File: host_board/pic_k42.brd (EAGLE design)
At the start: 55.6 x 67.3 mm, 40 parts, among them IC1 PIC18F57K42-E_PT, IC2 REF3440IDBVR, IC3 MAX232, K1 G6K-2P, Q1 ASF1, X1 332-02, X2 332-02, X3 332-02, X4 22-23-2101, X5 22-23-2101, X6 22-23-2101, X7 22-23-2101

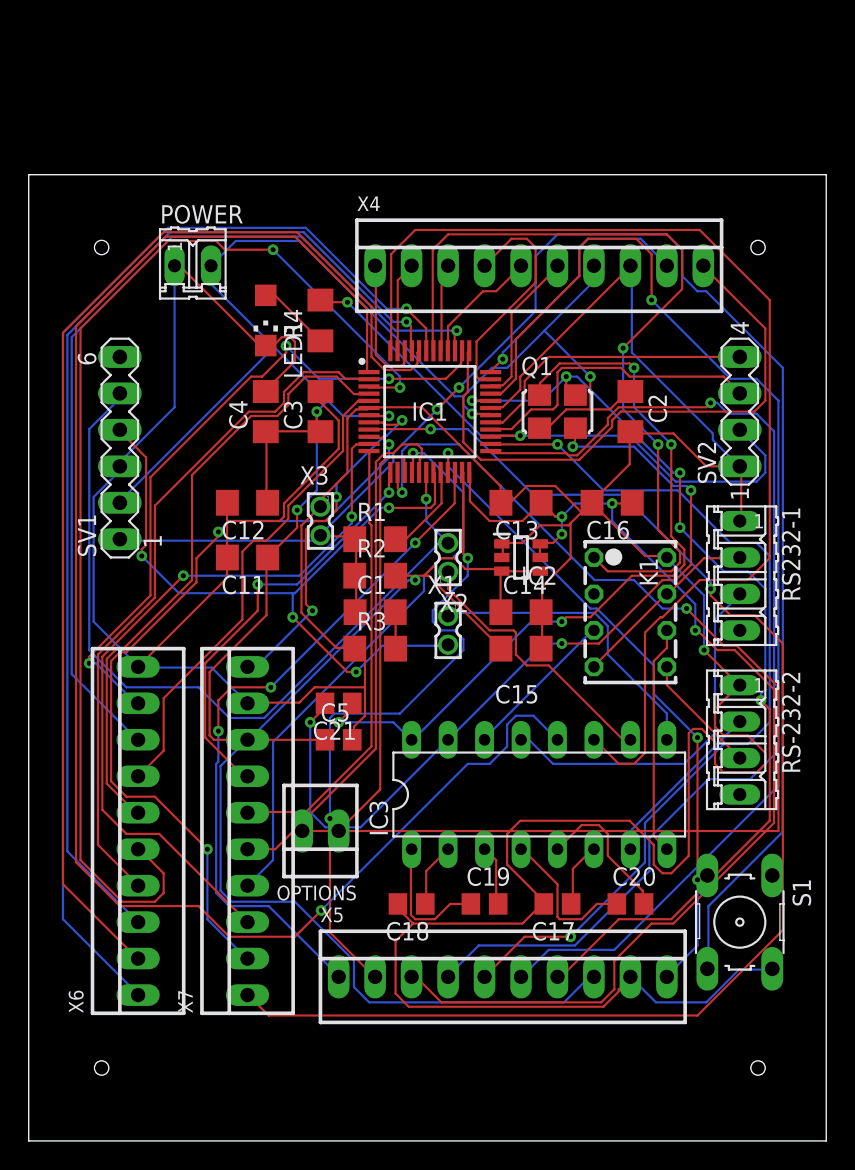
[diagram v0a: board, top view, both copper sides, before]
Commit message: update
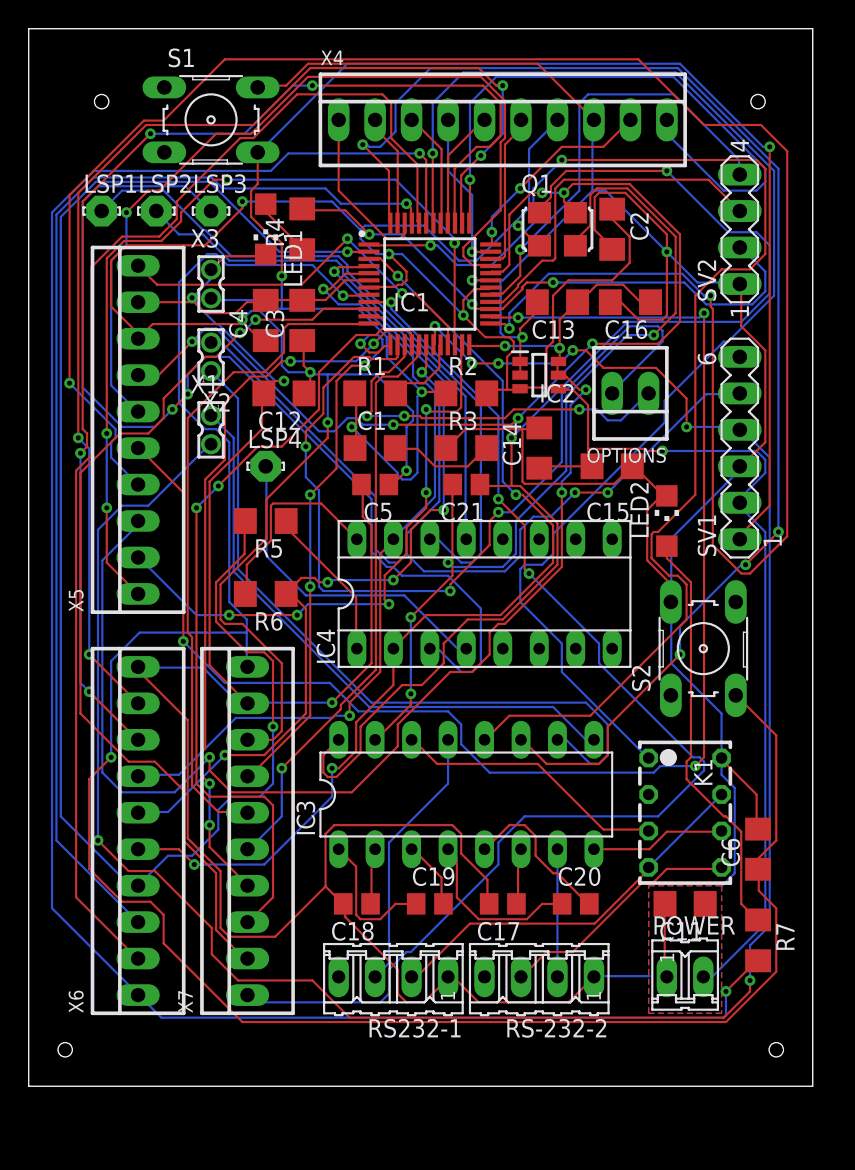
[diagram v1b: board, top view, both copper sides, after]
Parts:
- added C6: 0.1, rcl:C1206
- added IC4: ILAMP, ic-package:SOCKET-16
- added LED2: MODE, led:CHIPLED_1206
- added LSP1, LSP2, LSP3, LSP4: LSP10, solpad:LSP10
- added R5, R6, R7: 220, rcl:R1206
- added S2: MODESW, switch-omron:B3F-10XX
- S1: value (none) -> RESETSW
- moved S1 66.9 mm to (36.8, 62.2), turned to 0 degrees
- moved POWER 60.2 mm to (69.8, 2.54)
- moved X5 45.8 mm to (31.8, 40.6), turned to 90 degrees
- moved SV1 43.2 mm to (73.7, 39.4)
- moved C11 38.9 mm to (69.8, 7.62)
- moved OPTIONS 37.4 mm to (66.0, 43.2)
- moved RS232-1 36.9 mm to (49.5, 2.54), turned to 180 degrees
- moved X1 21.6 mm to (36.8, 40.6)
- moved X2 21.6 mm to (36.8, 45.7)
- moved RS-232-2 21.6 mm to (59.7, 2.54), turned to 180 degrees
- moved X3 18.2 mm to (36.8, 50.8)
- moved C5 18.0 mm to (48.3, 36.8), turned to 180 degrees
- moved C21 17.6 mm to (54.6, 36.8)
- moved R3 15.3 mm to (54.6, 39.4)
- moved K1 14.5 mm to (69.8, 15.2)
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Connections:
- new net N$17: IC4.1, R5.1
- new net N$55: IC4.14, LSP1.MP
- new net N$63: IC4.16, R6.2
- new net N$64: LED2.A, R7.1
- new net N$65: IC4.13, LSP2.MP
- new net N$67: IC4.3, LSP3.MP
- new net N$68: IC4.4, LSP4.MP
- net N$43: now also C6.1, IC1.8, S2.3, X7.10; no longer IC1.43, X6.1
- net N$46: now also R5.2
- net N$47: now also IC4.2
- net N$48: now also R6.1
- net N$49: now also IC4.15
- net N$52: now also IC1.43, R7.2, X6.1; no longer IC1.8, X7.10
- net VSS: now also C6.2, LED2.C, S2.2
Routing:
- net N$52: track 25.4 -> 135.8 mm, vias 3 -> 2
- net N$6: track 50.9 -> 152.5 mm, vias 4 -> 7
- net N$36: track 75.5 -> 148.6 mm, vias 1 -> 3
- net N$67: track 0.00 -> 72.5 mm, vias 0 -> 2
- net N$43: track 81.1 -> 146.2 mm, vias 1 -> 2
- net N$46: track 48.7 -> 108.3 mm, vias 0 -> 2
- net N$55: track 0.00 -> 48.3 mm
- net N$35: track 63.1 -> 102.1 mm, vias 2 -> 4
- net N$65: track 0.00 -> 37.2 mm
- net N$50: track 47.4 -> 81.7 mm, vias 3 -> 4
- net N$22: track 19.1 -> 51.4 mm
- net N$28: track 57.1 -> 88.7 mm, vias 2 -> 1
- net VCC: track 54.6 -> 85.4 mm, vias 4 -> 2
- net N$64: track 0.00 -> 29.0 mm
- net VSS: track 321.4 -> 347.2 mm, vias 1 -> 6
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- added copper zone on layer 1, net VDD
- added copper zone on layer 16, net VSS
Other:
- board size 55.6 x 67.3 mm -> 54.6 x 73.7 mm
